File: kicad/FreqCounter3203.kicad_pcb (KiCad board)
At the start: 2 copper layers, 30 x 40 mm, 25 parts, among them J1 max4466_Mic_Module, J2 WCH-LINKE, SW1 OK, SW2 ↓, SW3 ↑, SW7 SWITCH_INV, U1 SEEED_GROVE, U2 OLED_0.96in_SPI, U3 CH32V003F4P6, Y1 24M

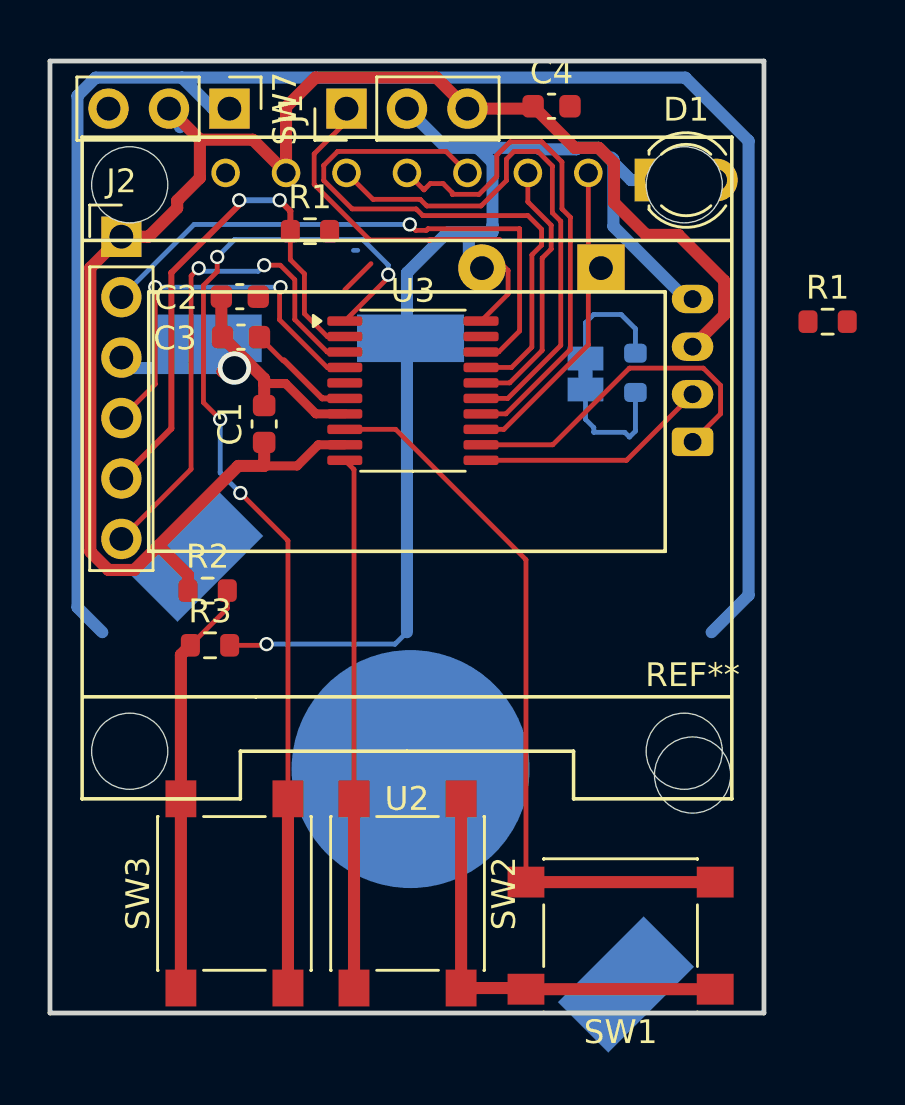
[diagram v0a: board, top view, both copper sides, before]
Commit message: change kicad files
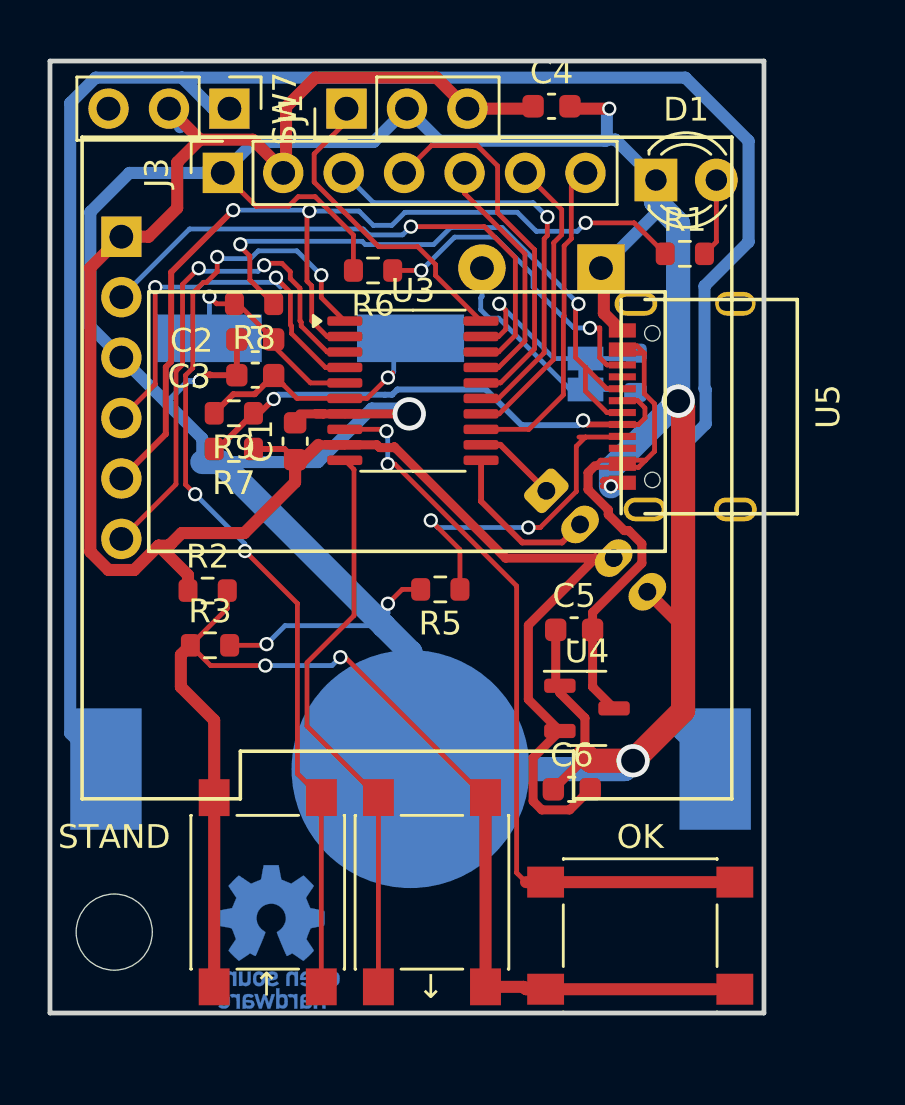
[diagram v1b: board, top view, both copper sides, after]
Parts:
- removed the R1 at (139.0, 44.4)
- removed the R1 at (160.8, 48.2)
- removed the REF** at (155.1, 67.2)
- removed U2: OLED_0.96in_SPI, library:OLED_0.96in_SPI
- added C5: 10u, Capacitor_SMD:C_0603_1608Metric, F.Cu at (150.1, 61.1)
- added C6: 1u, Capacitor_SMD:C_0603_1608Metric, F.Cu at (150.0, 67.8)
- added J3: Conn_01x07_Socket, Connector_PinSocket_2.54mm:PinSocket_1x07_P2.54mm_Vertical, F.Cu at (135.3, 41.9)
- added R1: 180Ω, Resistor_SMD:R_0603_1608Metric, F.Cu at (154.8, 45.3)
- added R5: 5.1k, Resistor_SMD:R_0603_1608Metric, F.Cu at (144.5, 59.4)
- added R6: 5.1k, Resistor_SMD:R_0603_1608Metric, F.Cu at (141.7, 46.0)
- added R7: 1.5k, Resistor_SMD:R_0603_1608Metric, F.Cu at (135.8, 53.5)
- added R8: 47, Resistor_SMD:R_0603_1608Metric, F.Cu at (136.7, 47.4)
- added R9: 47, Resistor_SMD:R_0603_1608Metric, F.Cu at (135.8, 52.0)
- added REF**: OSHW-Logo_5.7x6mm_Copper, Symbol:OSHW-Logo_5.7x6mm_Copper, B.Cu at (137.4, 74.0)
- added STAND: MountingHole_3mm, MountingHole:MountingHole_3mm, F.Cu at (130.8, 73.8)
- added U4: XC6206PxxxMR, Package_TO_SOT_SMD:SOT-23-3, F.Cu at (150.6, 64.4)
- added U5: USB-C_16PIN, library:USB_Type_C_16Pin_Female, F.Cu at (156.3, 51.8)
- J2: moved to B.Cu
- moved U1 6.48 mm to (148.9, 55.3), turned to -45 degrees
- moved C2 1.91 mm to (136.7, 48.9)
- moved C3 1.71 mm to (136.7, 50.4)
- moved C1 1.49 mm to (138.4, 53.2)
- moved SW3 1.40 mm to (137.2, 72.2)
- moved SW2 1.03 mm to (144.1, 72.2)
- moved SW1 0.83 mm to (152.9, 74.0)
- turned BT1 to 0 degrees
- turned J2 to 180 degrees
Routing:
- net GND: track 66.8 -> 162.5 mm, vias 2 -> 9
- net Net-(U5-DP1): track 0.00 -> 26.8 mm, vias 0 -> 2
- net +5V: track 0.00 -> 23.9 mm
- net Net-(U5-DN1): track 0.00 -> 21.5 mm, vias 0 -> 2
- net Net-(J2-Pin_5): track 22.7 -> 39.5 mm, vias 2 -> 3
- net Net-(R2-Pad2): track 36.2 -> 51.0 mm, vias 0 -> 2
- net Net-(U5-CC1): track 0.00 -> 14.6 mm, vias 0 -> 2
- net Net-(J3-Pin_5): track 24.9 -> 10.4 mm
- net +3V3: track 73.9 -> 88.3 mm
- net Net-(U5-CC2): track 0.00 -> 13.6 mm, vias 0 -> 2
- net Net-(BT1-Pad1): track 76.4 -> 89.5 mm
- net Net-(U1-Yellow/Dn/An/RX/SCL): track 14.6 -> 3.55 mm
- net Net-(J3-Pin_6): track 21.8 -> 12.6 mm
- net Net-(U3-PA1/OSCI/A1/T1CH2/OPN0): track 0.37 -> 9.12 mm, vias 0 -> 1
- net Net-(U3-PA2/OSCO/A0/T1CH2N/OPP0/AETR2_): track 4.64 -> 11.5 mm, vias 0 -> 1
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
